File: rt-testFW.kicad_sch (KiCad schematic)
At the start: 13 parts, among them J1 1Min, J2 2Min, J3 3Min, J4 5Min, SW1 TestStart-Peach, SW2 Reset-Black

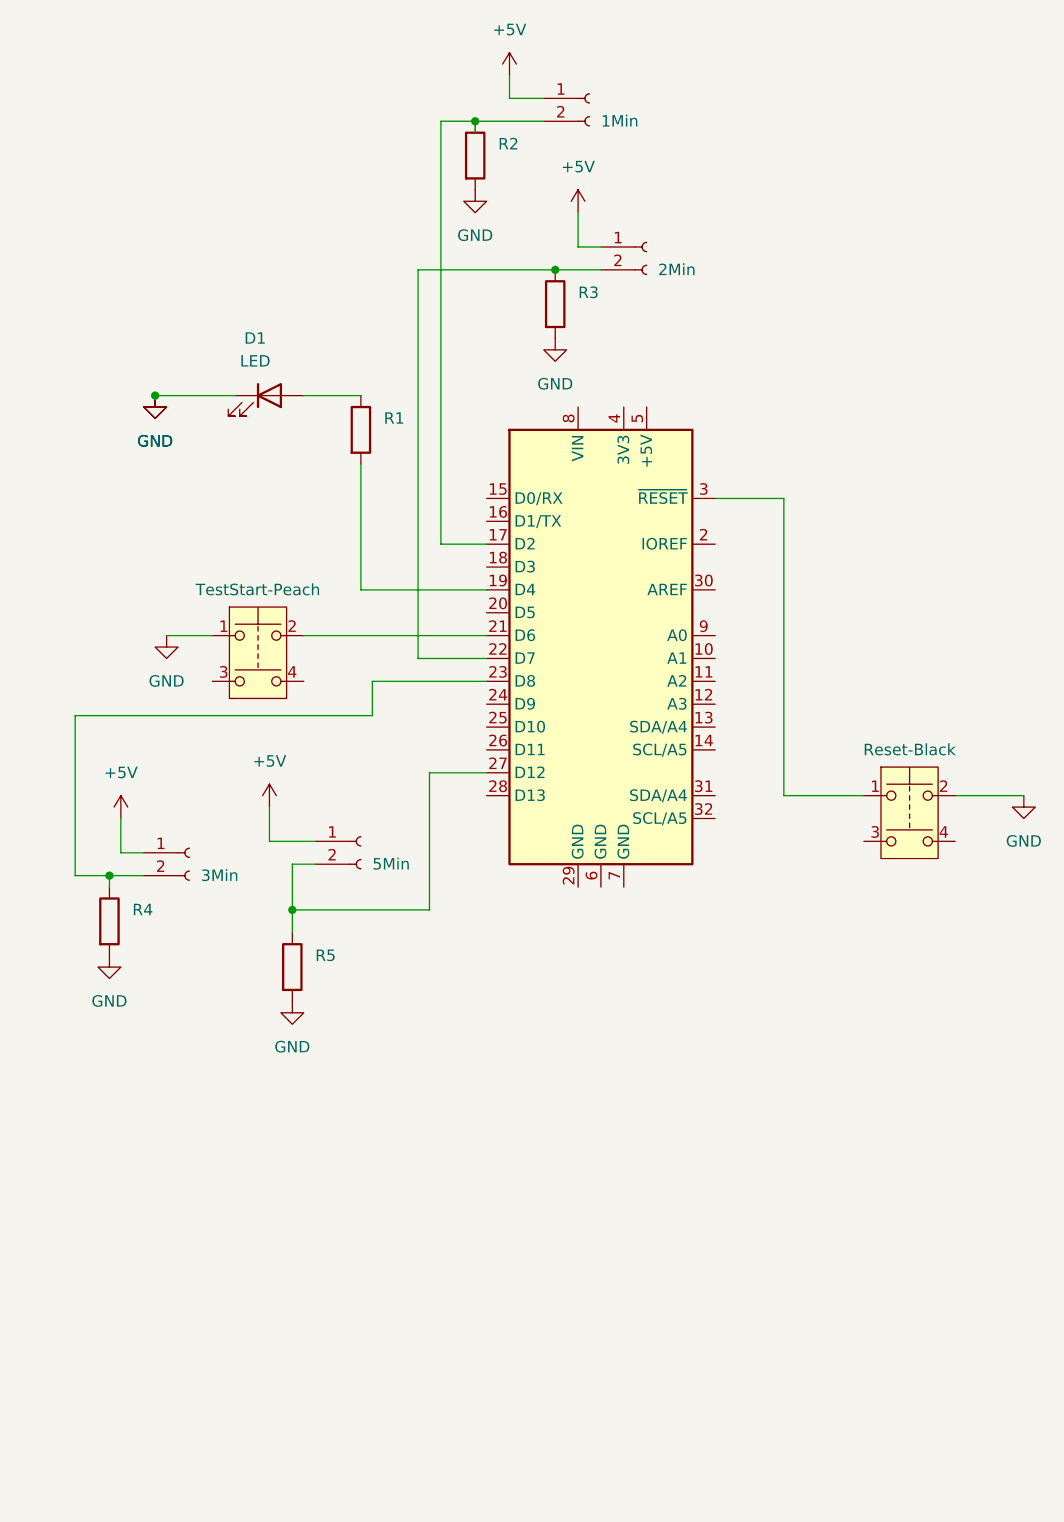
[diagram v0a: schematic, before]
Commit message: initial iteration complete
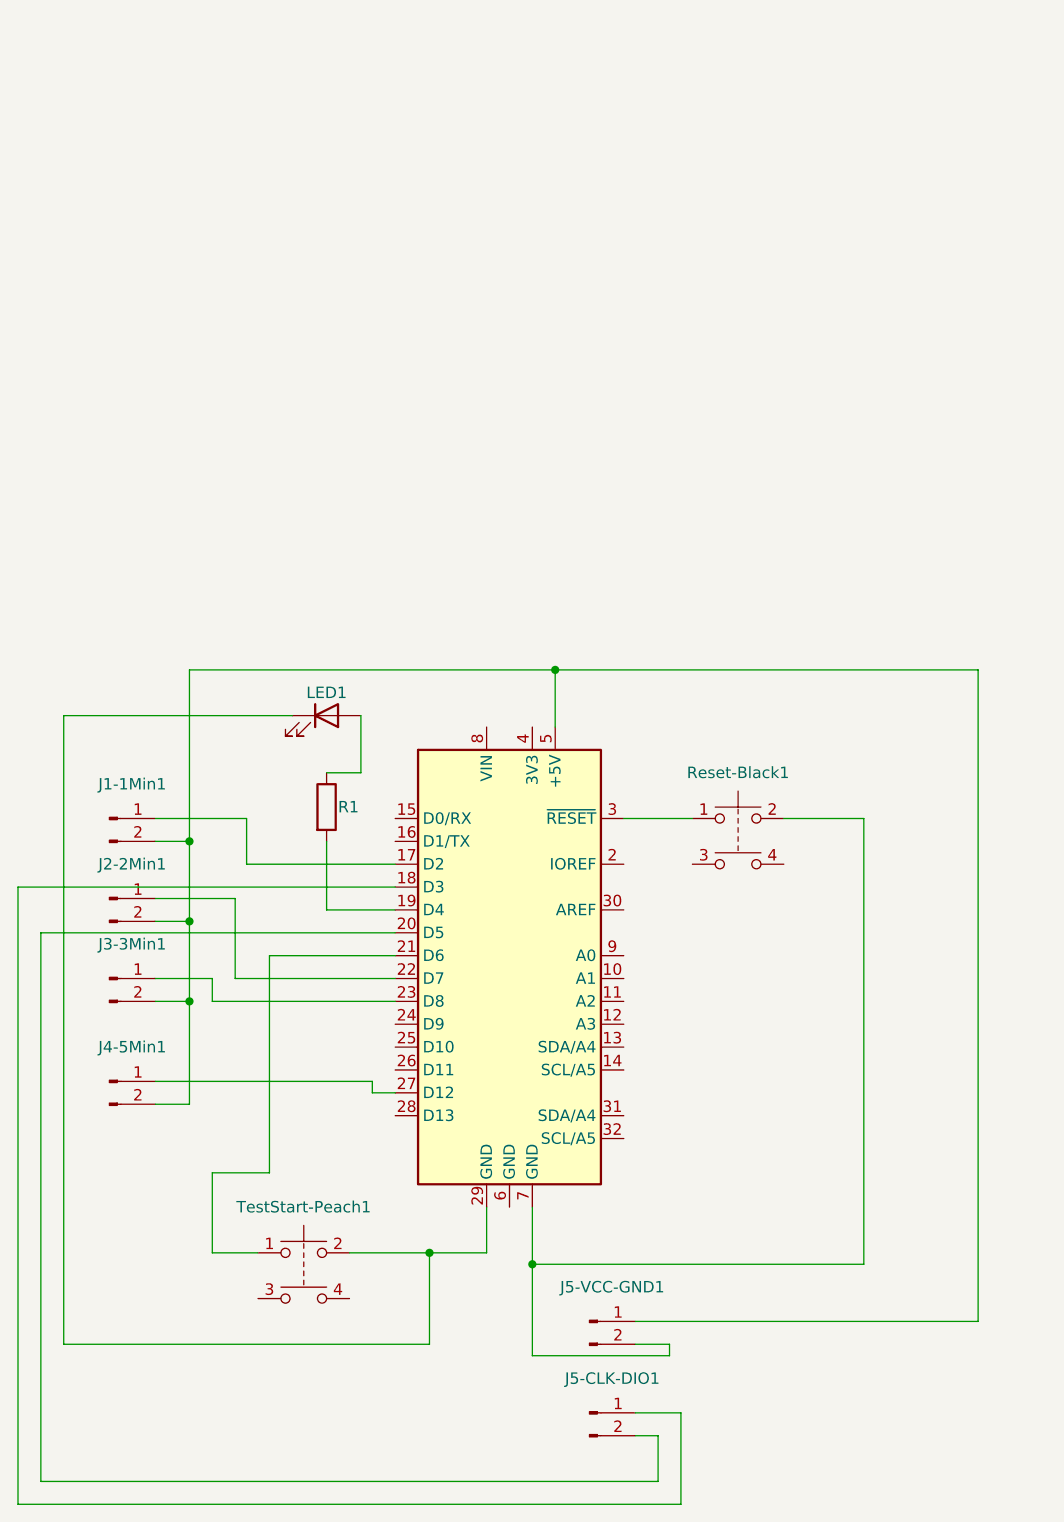
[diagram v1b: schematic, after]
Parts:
- removed D1: LED, LED_THT:LED_D4.0mm, symbol Device:LED
- removed J1: 1Min, Connector_PinSocket_2.54mm:PinSocket_1x02_P2.54mm_Vertical, symbol Connector:Conn_01x02_Socket
- removed J2: 2Min, Connector_PinSocket_2.54mm:PinSocket_1x02_P2.54mm_Vertical, symbol Connector:Conn_01x02_Socket
- removed J3: 3Min, Connector_PinSocket_2.54mm:PinSocket_1x02_P2.54mm_Vertical, symbol Connector:Conn_01x02_Socket
- removed J4: 5Min, Connector_PinSocket_2.54mm:PinSocket_1x02_P2.54mm_Vertical, symbol Connector:Conn_01x02_Socket
- removed R2, R3, R4, R5: R, Resistor_THT:R_Axial_DIN0309_L9.0mm_D3.2mm_P2.54mm_Vertical, symbol Device:R
- removed SW1: TestStart-Peach, Button_Switch_THT:SW_PUSH_6mm, symbol Switch:SW_Push_Dual
- removed SW2: Reset-Black, Button_Switch_THT:SW_PUSH_6mm, symbol Switch:SW_Push_Dual
- added J1-1Min1, J2-2Min1, J3-3Min1, J4-5Min1, J5-CLK-DIO1, J5-VCC-GND1: Conn_01x02_Male, Connector_PinHeader_2.00mm:PinHeader_1x02_P2.00mm_Vertical, symbol Connector:Conn_01x02_Male
- added LED1: LED, Connector_PinHeader_2.00mm:PinHeader_1x02_P2.00mm_Vertical, symbol Device:LED
- added Reset-Black1, TestStart-Peach1: SW_Push_Dual, Button_Switch_THT:SW_PUSH_6mm, symbol Switch:SW_Push_Dual
- R1: footprint Resistor_THT:R_Axial_DIN0309_L9.0mm_D3.2mm_P2.54mm_Vertical -> Connector_PinHeader_2.00mm:PinHeader_1x02_P2.00mm_Vertical
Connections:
- net at R1.1: now also LED1.2 (A)
- net at A1.23 (D8): now also J3-3Min1.1 (Pin_1)
- net at A1.17 (D2): now also J1-1Min1.1 (Pin_1)
- net at A1.22 (D7): now also J2-2Min1.1 (Pin_1)
- net at A1.21 (D6): now also TestStart-Peach1.1
- net at A1.27 (D12): now also J4-5Min1.1 (Pin_1)
- net at A1.18 (D3): now also J5-CLK-DIO1.1 (Pin_1)
- net at A1.20 (D5): now also J5-CLK-DIO1.2 (Pin_2)
- net at A1.29 (GND): now also LED1.1 (K), TestStart-Peach1.2
- net at A1.3 (~{RESET}): now also Reset-Black1.1
- net at A1.5 (+5V): now also J1-1Min1.2 (Pin_2), J2-2Min1.2 (Pin_2), J3-3Min1.2 (Pin_2), J4-5Min1.2 (Pin_2), J5-VCC-GND1.1 (Pin_1)
- net at A1.7 (GND): now also J5-VCC-GND1.2 (Pin_2), Reset-Black1.2
